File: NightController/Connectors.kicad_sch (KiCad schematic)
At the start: 2 parts, among them J201 Conn_02x20_Odd_Even, J202 Conn_02x20_Odd_Even

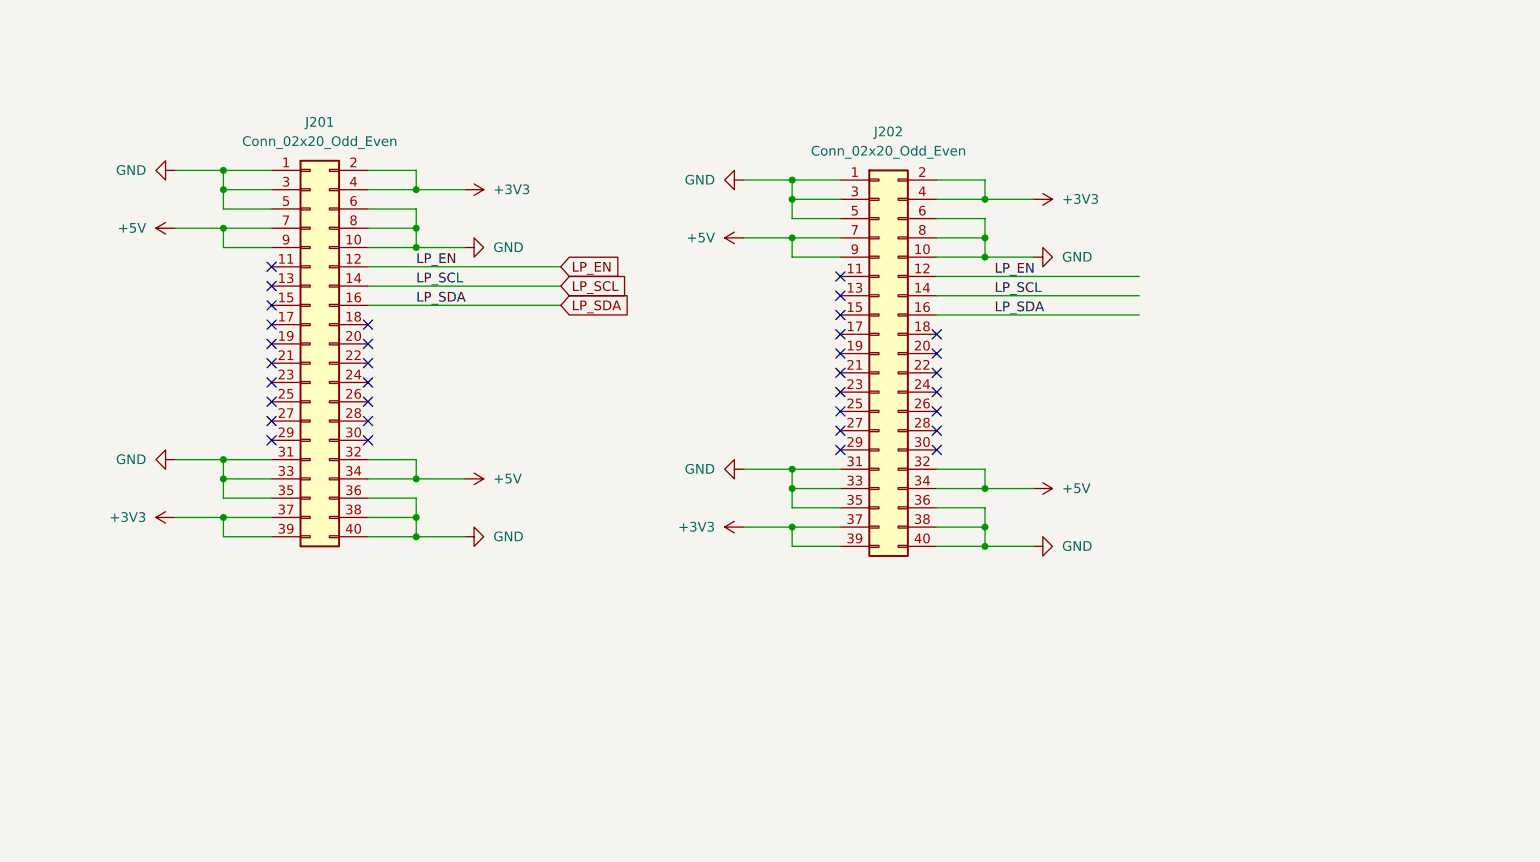
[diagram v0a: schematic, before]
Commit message: Working on files
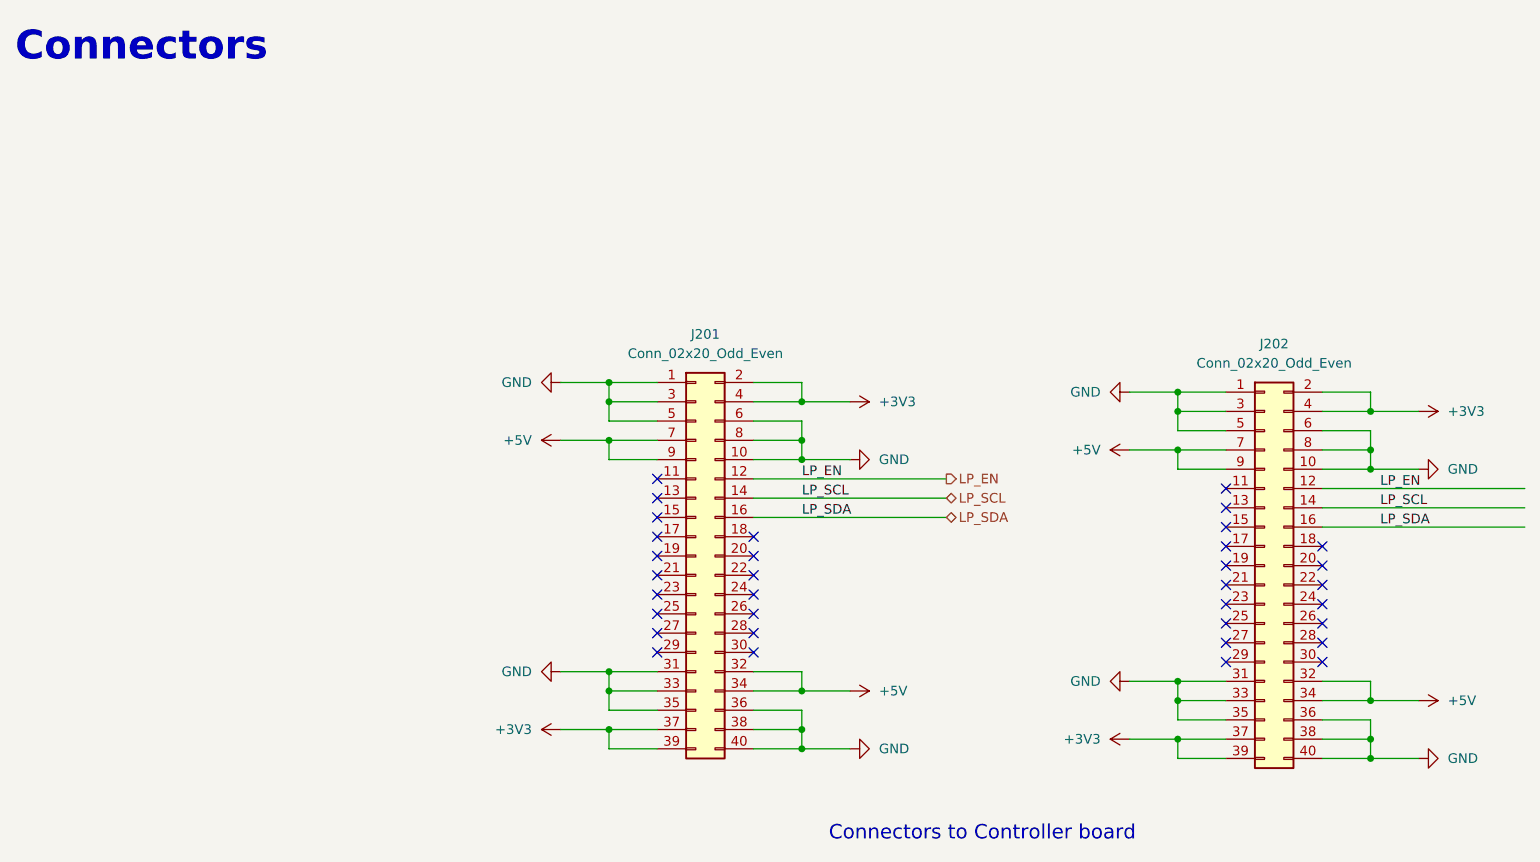
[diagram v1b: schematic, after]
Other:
- note added: "Connectors"
- note added: "Connectors to Controller board"
- title: (none) -> NightLight
- moved on the sheet: J201, J202
